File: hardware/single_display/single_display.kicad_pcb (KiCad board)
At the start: 2 copper layers, 16 x 34.3 mm, 11 parts, among them J1 Conn_01x05_Male, J2 Conn_01x05_Male, U1 KCSC02-123

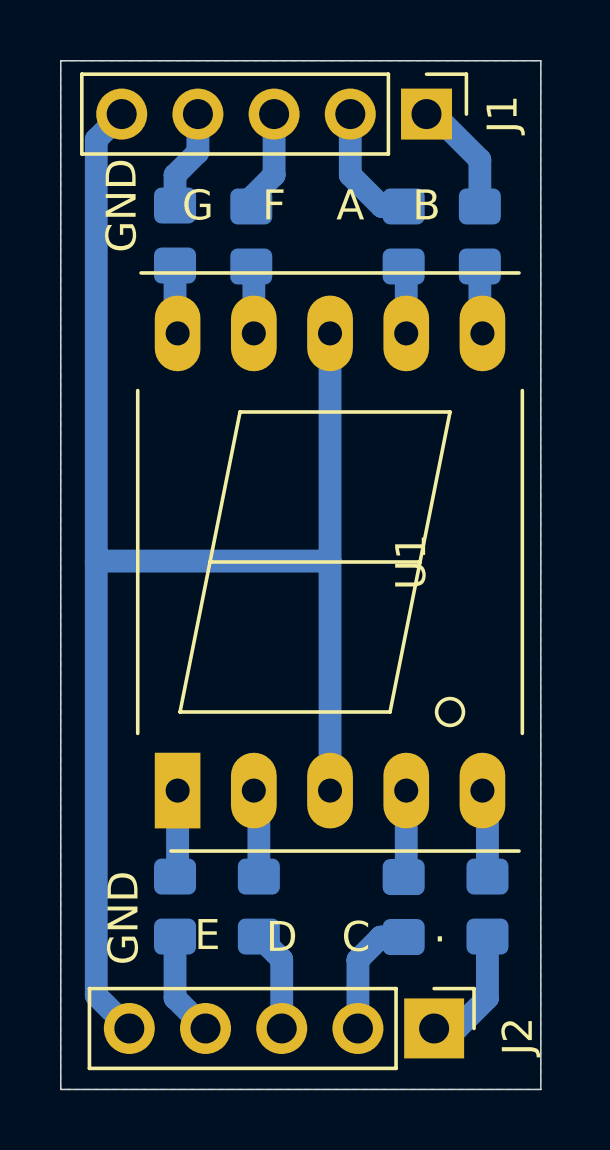
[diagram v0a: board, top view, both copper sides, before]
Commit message: Projeto em kicad 6
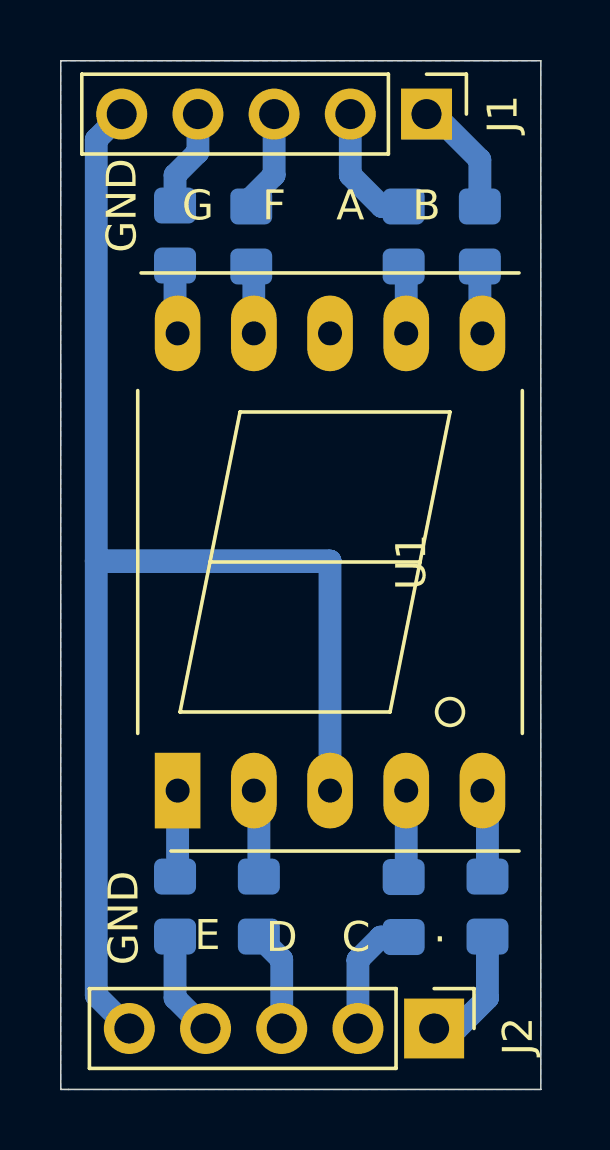
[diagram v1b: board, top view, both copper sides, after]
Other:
- net class Default removed
